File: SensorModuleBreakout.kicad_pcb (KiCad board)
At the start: 2 copper layers, 41 x 42.7 mm, 23 parts, among them J1 Conn_01x04, J2 Conn_ST_STDC14, J3 Conn_01x03, J4 Conn_01x10, J5 Conn_01x15, U1 STM32U031C8Tx

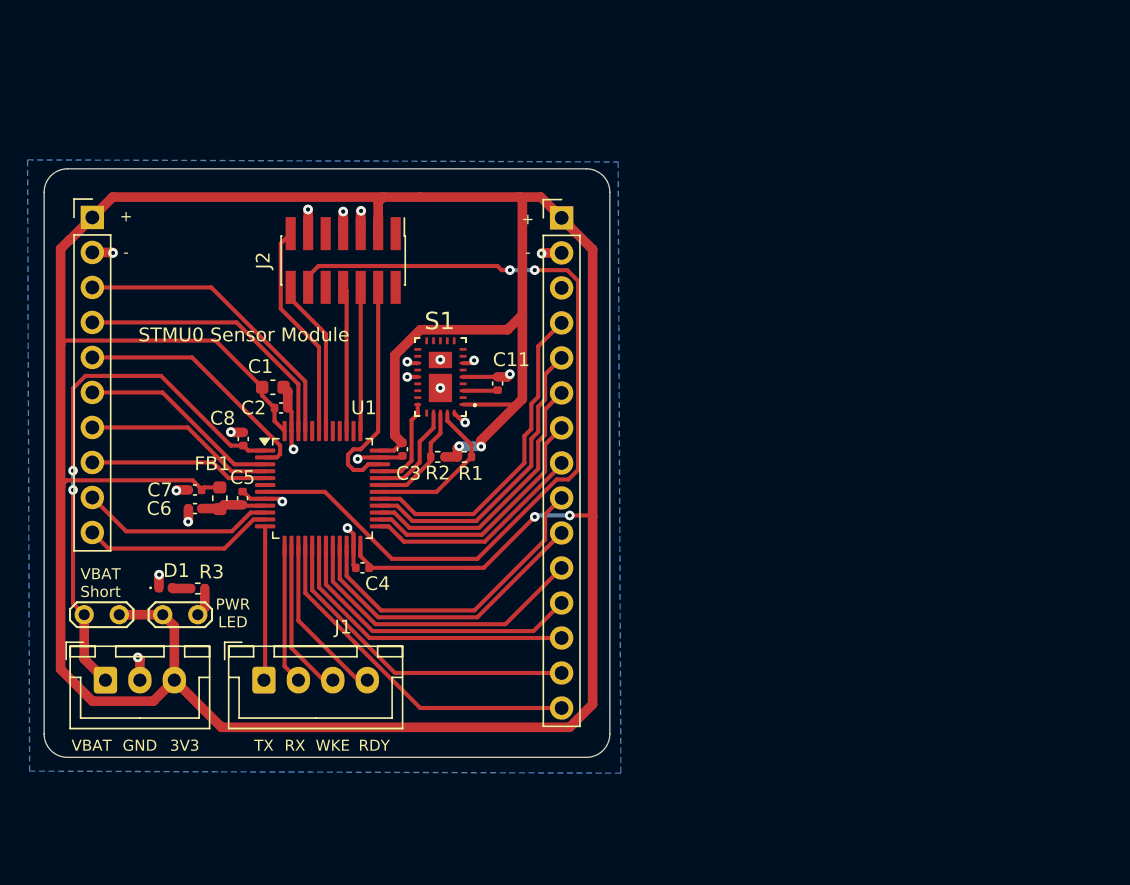
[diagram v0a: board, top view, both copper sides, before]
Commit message: V2
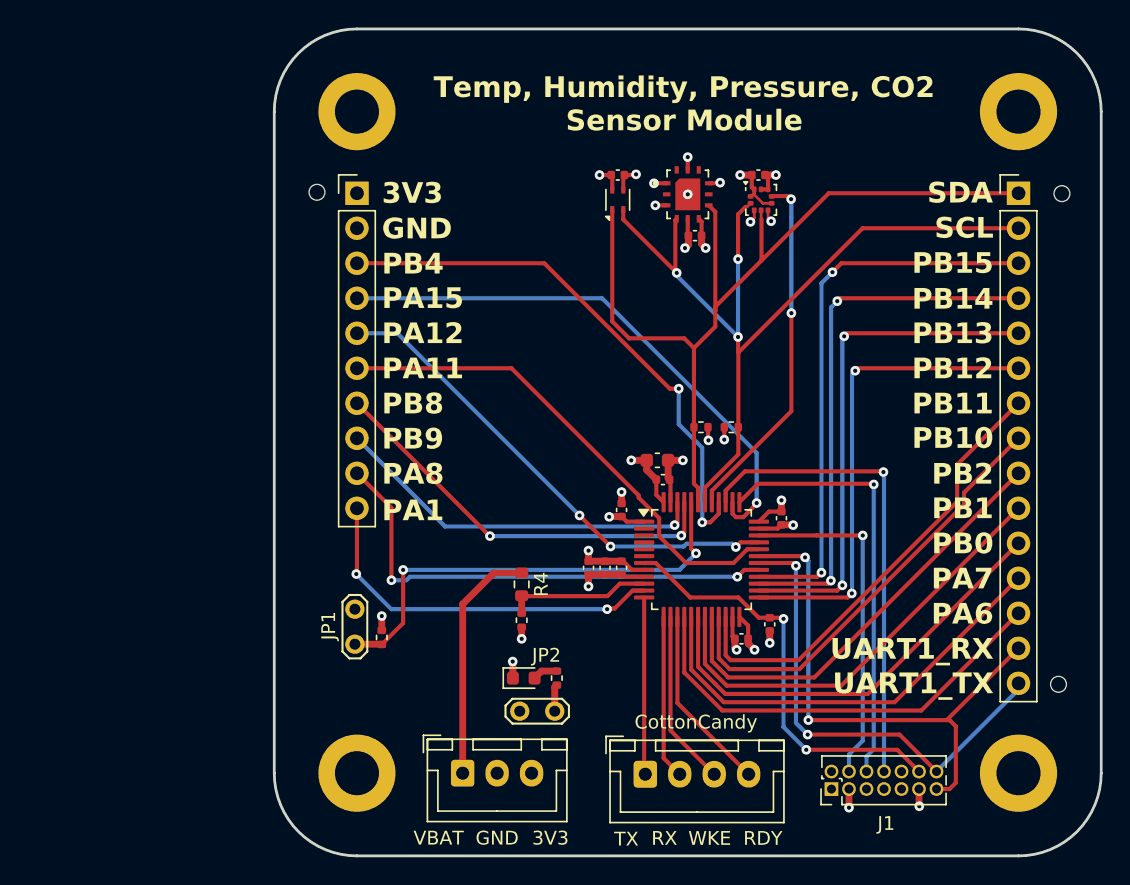
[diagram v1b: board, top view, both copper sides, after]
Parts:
- removed FB1: 120R, Inductor_SMD:L_0603_1608Metric
- removed S1: USEQGSEAC82180, USEQGS:USEQGSEAC82180
- added C10: 100n, Capacitor_SMD:C_0402_1005Metric, F.Cu at (130.5, 65.0)
- added C12: 100n, Capacitor_SMD:C_0402_1005Metric, F.Cu at (135.9, 93.2)
- added C9: 100n, Capacitor_SMD:C_0402_1005Metric, F.Cu at (124.9, 60.6)
- added H1: MountingHole_Pad, MountingHole:MountingHole_3.2mm_M3_DIN965_Pad, F.Cu at (106.0, 56.0)
- added H2: MountingHole_Pad, MountingHole:MountingHole_3.2mm_M3_DIN965_Pad, F.Cu at (154.0, 56.0)
- added H3: MountingHole_Pad, MountingHole:MountingHole_3.2mm_M3_DIN965_Pad, F.Cu at (106.0, 104.0)
- added H4: MountingHole_Pad, MountingHole:MountingHole_3.2mm_M3_DIN965_Pad, F.Cu at (154.0, 104.0)
- added R4: 2M, Resistor_SMD:R_0603_1608Metric, F.Cu at (118.0, 90.3)
- added R5: 1M, Resistor_SMD:R_0402_1005Metric, F.Cu at (118.0, 92.9)
- added R6: 220r, Resistor_SMD:R_0402_1005Metric, F.Cu at (120.5, 97.1)
- added REF**: ToolingHole_1.152mm, MountingHole:ToolingHole_1.152mm, F.Cu at (157.2, 62.0)
- added REF**: ToolingHole_1.152mm, MountingHole:ToolingHole_1.152mm, F.Cu at (103.1, 61.9)
- added REF**: ToolingHole_1.152mm, MountingHole:ToolingHole_1.152mm, F.Cu at (156.9, 97.5)
- added U2: SHT4x, Sensor_Humidity:Sensirion_DFN-4_1.5x1.5mm_P0.8mm_SHT4x_NoCentralPad, F.Cu at (124.9, 62.4)
- added U3: STC31-C-R3, STC31_C_R3:XDCR_STC31-C-R3, F.Cu at (130.0, 62.0)
- added U4: LPS22DF, Package_LGA:ST_HLGA-10_2x2mm_P0.5mm_LayoutBorder3x2y, F.Cu at (135.3, 62.4)
- C5: value 10n -> 100n
- C6: value 1u -> 10n
- C8: value 100n -> 1u
- D1: footprint LED_SMD:LED_0402_1005Metric -> LED_SMD:LED_0603_1608Metric
- J1: value Conn_01x04 -> Conn_ST_STDC14; footprint Connector_JST:JST_XH_B4B-XH-A_1x04_P2.50mm_Vertical -> Connector_PinHeader_1.27mm:PinHeader_2x07_P1.27mm_Vertical
- J2: value Conn_ST_STDC14 -> Conn_01x10; footprint Connector_PinHeader_1.27mm:PinHeader_2x07_P1.27mm_Vertical_SMD -> Connector_PinHeader_2.54mm:PinHeader_1x10_P2.54mm_Vertical
- J3: value Conn_01x03 -> Conn_01x15; footprint Connector_JST:JST_XH_B3B-XH-A_1x03_P2.50mm_Vertical -> Connector_PinHeader_2.54mm:PinHeader_1x15_P2.54mm_Vertical
- J4: value Conn_01x10 -> Conn_01x03; footprint Connector_PinHeader_2.54mm:PinHeader_1x10_P2.54mm_Vertical -> Connector_JST:JST_XH_B3B-XH-A_1x03_P2.50mm_Vertical
- J5: value Conn_01x15 -> Conn_01x04; footprint Connector_PinHeader_2.54mm:PinHeader_1x15_P2.54mm_Vertical -> Connector_JST:JST_XH_B4B-XH-A_1x04_P2.50mm_Vertical
- JP1: value JP -> Jumper_2_Open
- JP2: value Jumper_2_Open -> JP
- R1, R2, R3: value 1k5 -> 10k
- moved J3 75.1 mm to (154.0, 61.9)
- moved J4 48.5 mm to (113.7, 104.0)
- moved J1 41.9 mm to (140.4, 105.2), turned to 90 degrees
- moved J5 40.8 mm to (126.9, 104.1)
- moved R3 38.3 mm to (131.0, 78.9), turned to 180 degrees
- moved JP2 32.4 mm to (120.3, 99.5)
- moved C6 31.2 mm to (125.2, 89.1), turned to 90 degrees
- moved C7 30.3 mm to (124.0, 89.1), turned to 90 degrees
- moved C1 28.4 mm to (127.8, 81.3)
- moved C2 28.2 mm to (128.2, 82.7)
- moved U1 28.0 mm to (131.0, 88.5)
- moved C4 28.0 mm to (133.9, 94.2)
- moved C3 28.0 mm to (136.8, 85.5)
- moved C5 27.5 mm to (125.2, 84.9)
- moved D1 26.8 mm to (118.1, 97.1)
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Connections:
- C11 pad 1: Net-(S1-CAP) -> +3V3
- C5 pad 1: +3V3A -> +3V3
- C6 pad 1: +3V3A -> +3V3
- C8 pad 1: VBAT -> +3V3
- J1 pad 1: TX -> unconnected-(J1-NC-Pad1)
- J1 pad 2: RX -> unconnected-(J1-NC-Pad2)
- J1 pad 3: WKE -> +3V3
- J1 pad 4: RDY -> JTMS/SWDIO
- J2 pad 1: unconnected-(J2-NC-Pad1) -> +3V3
- J2 pad 10: unconnected-(J2-JTDI/NC-Pad10) -> PA1
- J2 pad 2: unconnected-(J2-NC-Pad2) -> GND
- J2 pad 3: +3V3 -> PB4
- J2 pad 4: JTMS/SWDIO -> PA15
- J2 pad 5: GND -> PA12
- J2 pad 6: JTCK_SWCLK -> PA11
- J2 pad 7: GND -> PB8
- J2 pad 8: JTDO/SWO -> PB9
- J2 pad 9: unconnected-(J2-JRCLK/NC-Pad9) -> PA8
- J3 pad 1: VBAT -> SDA
- J3 pad 2: GND -> SCL
- J3 pad 3: +3V3 -> PB15
- J4 pad 1: +3V3 -> VBAT
- J4 pad 3: PB8 -> +3V3
- J5 pad 1: +3V3 -> CC_TX
- J5 pad 2: GND -> CC_RX
- J5 pad 3: unconnected-(J5-Pin_3-Pad3) -> CC_WKE
- J5 pad 4: PA8 -> CC_RDY
- JP1 pad 1: Net-(JP1-A) -> +3V3
- JP1 pad 2: +3V3 -> /BOOT0
- JP2 pad 1: +3V3 -> Net-(JP2-A)
- JP2 pad 2: VBAT -> +3V3
- R1 pad 1: +3V3 -> /BOOT0
- R1 pad 2: SCL -> GND
- R2 pad 2: SDA -> SCL
- R3 pad 1: Net-(D1-A) -> +3V3
- R3 pad 2: Net-(JP1-A) -> SDA
- U1 pad 1: VBAT -> +3V3
- U1 pad 10: PA0 -> Net-(U1-PA0)
- U1 pad 12: TX -> CC_TX
- U1 pad 13: RX -> CC_RX
- U1 pad 14: WKE -> CC_WKE
- U1 pad 15: RDY -> CC_RDY
- U1 pad 2: PC13 -> unconnected-(U1-PC13-Pad2)
- U1 pad 3: PC14 -> unconnected-(U1-PC14-Pad3)
- U1 pad 30: SCL -> VCP_TX
- U1 pad 31: SDA -> VCP_RX
- U1 pad 32: INT -> PA11
- U1 pad 33: CS -> PA12
- U1 pad 38: unconnected-(U1-PA15-Pad38) -> PA15
- U1 pad 4: PC15 -> unconnected-(U1-PC15-Pad4)
- U1 pad 40: unconnected-(U1-PB4-Pad40) -> PB4
- U1 pad 41: unconnected-(U1-PB5-Pad41) -> INT
- U1 pad 42: VCP_TX -> SCL
- U1 pad 43: VCP_RX -> SDA
- U1 pad 44: unconnected-(U1-PF3-Pad44) -> /BOOT0
- U1 pad 5: PF0 -> unconnected-(U1-PF0-Pad5)
- U1 pad 9: +3V3A -> +3V3
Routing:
- net +3V3: track 256.7 -> 30.0 mm, vias 4 -> 11
- net SDA: track 8.18 -> 66.7 mm
- net SCL: track 11.6 -> 64.1 mm, vias 0 -> 3
- net PA15: track 0.00 -> 40.4 mm, vias 0 -> 1
- net PB4: track 0.00 -> 39.8 mm, vias 0 -> 2
- net PA11: track 0.00 -> 36.3 mm
- net PA12: track 0.00 -> 35.9 mm, vias 0 -> 3
- net /BOOT0: track 0.00 -> 33.6 mm, vias 0 -> 2
- net NRST: track 64.1 -> 30.8 mm
- net JTDO/SWO: track 10.5 -> 34.7 mm, vias 0 -> 1
- net VCP_RX: track 15.8 -> 39.2 mm, vias 0 -> 2
- net VCP_TX: track 11.5 -> 34.7 mm, vias 0 -> 2
- net VBAT: track 38.9 -> 17.5 mm, vias 2 -> 0
- net JTCK_SWCLK: track 10.4 -> 31.4 mm, vias 0 -> 1
- net PB14: track 19.9 -> 39.0 mm, vias 0 -> 2
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- added copper zone on In2.Cu, net +3V3
- added copper zone on In1.Cu, net GND
- removed copper zone on B.Cu, net GND
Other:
- board size 41 x 42.7 mm -> 60 x 60 mm
- copper layers 2 -> 4
- board text added: "CottonCandy"
- board text added: "PA11"
- board text added: "PA12"
- board text added: "PA15"
- board text added: "PA6"
- board text added: "PB4"
- board text added: "SCL"
- board text added: "SDA"
- board text added: "Temp, Humidity, Pressure, CO2 Sensor Module"
- board text added: "UART1_RX"
- board text added: "UART1_TX"
- board text removed: "+"
- board text removed: "-"
- board text removed: "NC"
- board text removed: "PA0"
- board text removed: "PC13"
- board text removed: "PC14"
- board text removed: "PC15"
- board text removed: "PF0"
- board text removed: "PWR LED"
- board text removed: "STMU0 Sensor Module"
- board text removed: "VBAT Short"
